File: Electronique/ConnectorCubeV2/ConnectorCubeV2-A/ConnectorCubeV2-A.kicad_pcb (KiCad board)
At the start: 2 copper layers, 95.2 x 95.2 mm, 133 parts, among them J1001 Conn_02x20_Odd_Even, J1002 Conn_02x20_Odd_Even, J1003 Conn_01x03, J1004 Conn_01x03, J1005 Conn_01x03, J1006 Conn_01x03, J1007 Conn_01x03, J1008 Conn_01x03, J1009 Conn_01x03, J1010 Conn_01x03, J1011 Conn_01x03, J1012 Conn_01x03, J1013 Conn_01x03, J201 Conn_01x04, J202 Conn_01x04, J203 Conn_01x04, J301 Conn_02x08_Odd_Even, J302 Conn_02x10_Odd_Even, J401 Conn_01x03, J402 Conn_01x03, J403 Conn_01x03, J404 Conn_01x03, J405 Conn_01x03, J501 Conn_01x04, J601 Conn_01x06, J602 Conn_01x06, J603 Conn_01x06, J801 Conn_01x02, J802 Conn_01x02, J901 Conn_01x04, J902 Conn_01x04, J903 Conn_01x04, K701 CONN_3, K702 CONN_3, Q301 BSS123, Q302 BSS123, Q303 BSS123, Q304 BSS123, Q305 BS250, Q401 BSS123, Q402 BSS123, Q403 BSS123, Q404 BSS123, Q405 BSS123, Q601 BSS123, Q602 BSS123, Q603 BSS123, Q604 BSS123, Q605 BSS123, Q606 BSS123, Q901 BSS123, Q902 BSS123, Q903 BSS123, U201 PCA9306, U202 PCA9306, U203 PCA9306, U301 74LVCC3245

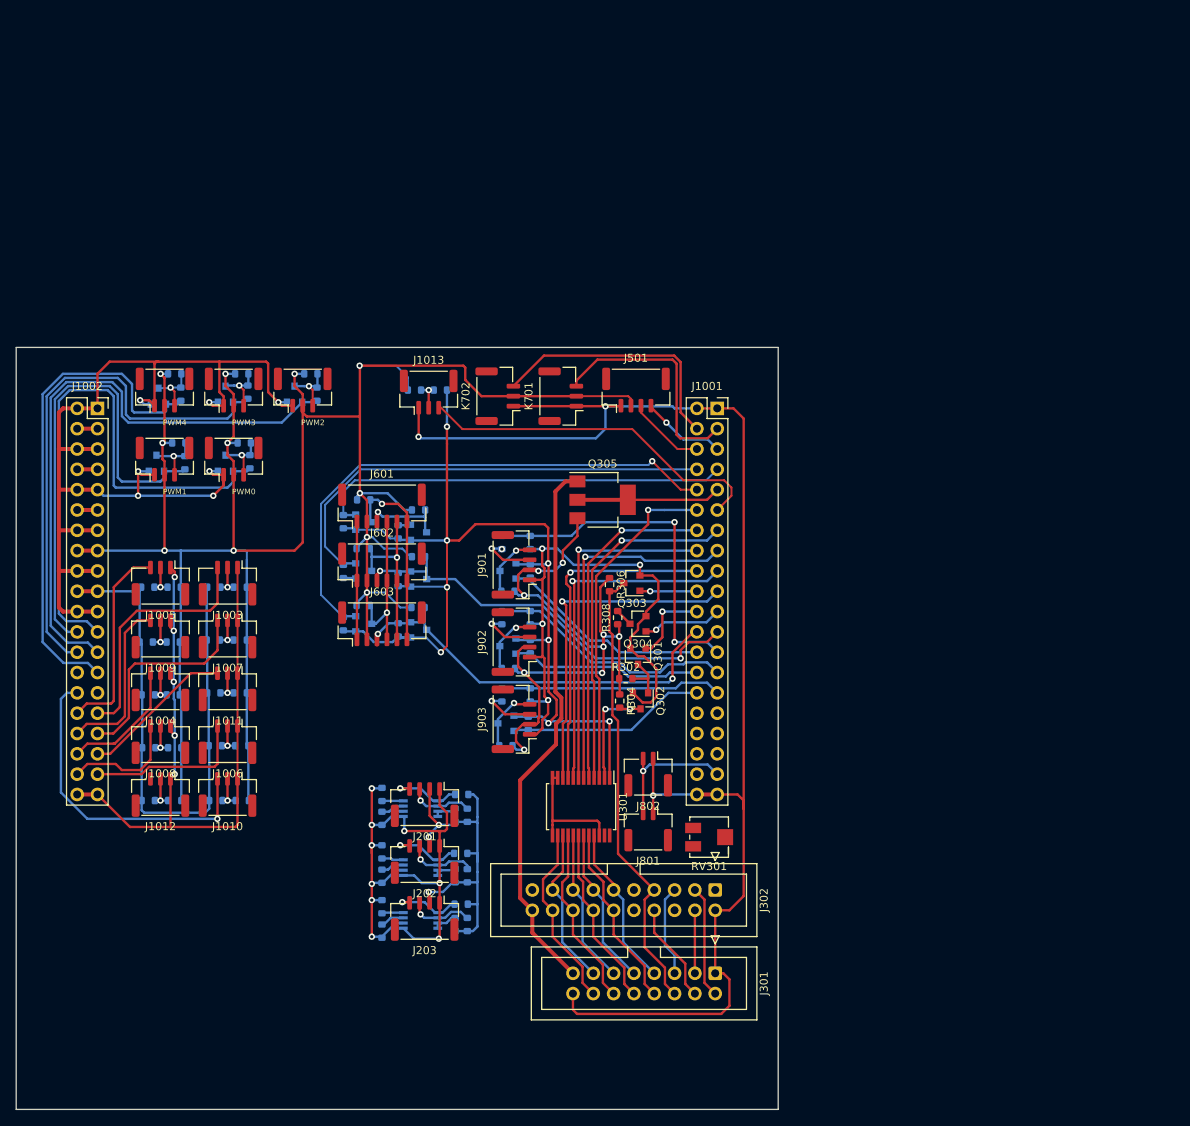
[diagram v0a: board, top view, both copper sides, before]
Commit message: CONNECTOR BOARD V2.00
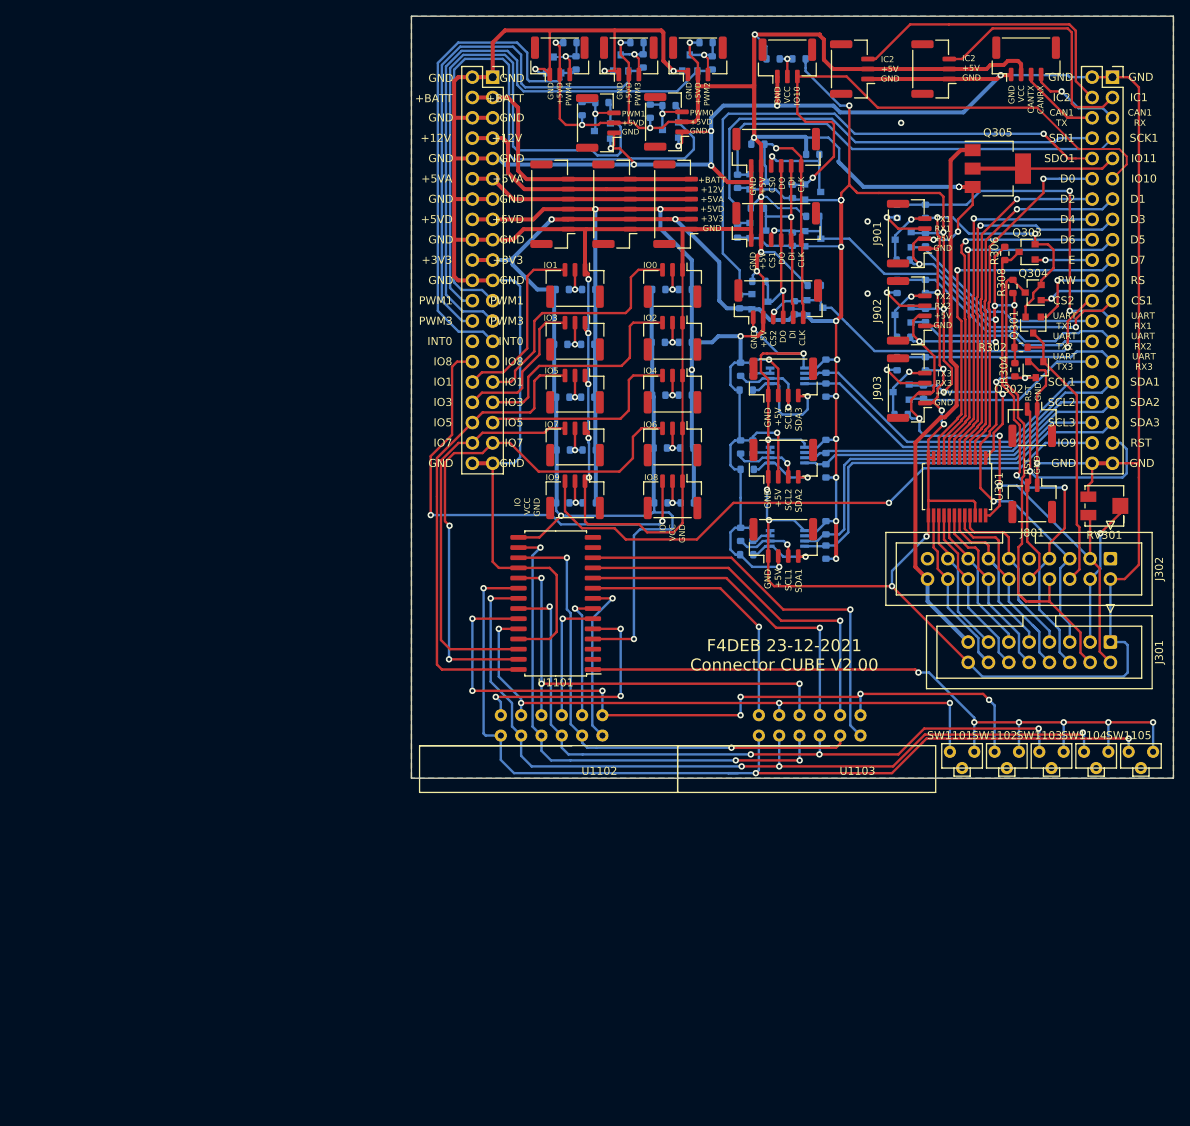
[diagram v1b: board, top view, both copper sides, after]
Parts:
- added J1201: Conn_01x06, Connector_JST:JST_GH_BM06B-GHS-TBT_1x06-1MP_P1.25mm_Vertical, F.Cu at (110.0, 75.3)
- added J1202: Conn_01x06, Connector_JST:JST_GH_BM06B-GHS-TBT_1x06-1MP_P1.25mm_Vertical, F.Cu at (117.7, 75.3)
- added J1203: Conn_01x06, Connector_JST:JST_GH_BM06B-GHS-TBT_1x06-1MP_P1.25mm_Vertical, F.Cu at (125.3, 75.3)
- added SW1101: SW_PUSH_SMALL, F4DEB-LIBRARY-KICAD5:BOUTON_SWITCH_4.5x4.5_angled, F.Cu at (159.6, 143.8)
- added SW1102: SW_PUSH_SMALL, F4DEB-LIBRARY-KICAD5:BOUTON_SWITCH_4.5x4.5_angled, F.Cu at (165.2, 143.8)
- added SW1103: SW_PUSH_SMALL, F4DEB-LIBRARY-KICAD5:BOUTON_SWITCH_4.5x4.5_angled, F.Cu at (170.8, 143.8)
- added SW1104: SW_PUSH_SMALL, F4DEB-LIBRARY-KICAD5:BOUTON_SWITCH_4.5x4.5_angled, F.Cu at (176.4, 143.8)
- added SW1105: SW_PUSH_SMALL, F4DEB-LIBRARY-KICAD5:BOUTON_SWITCH_4.5x4.5_angled, F.Cu at (182.0, 143.8)
- added U1101: TM1638, Package_SO:SOIC-28W_7.5x17.9mm_P1.27mm, F.Cu at (110.4, 125.2)
- added U1102: CA56-12EWA, F4DEB-LIBRARY-KICAD5:2841BS, F.Cu at (93.3, 143.0)
- added U1103: CA56-12EWA, F4DEB-LIBRARY-KICAD5:2841BS, F.Cu at (125.6, 143.0)
- R1001, R1002, R1003, R1004, R1005, R1007, R1009, R1010, R1011, R1012, R1013, R1014, R1015, R1016, R1017, R1018, R1019, R1020, R1021, R1022: value R -> 0
- moved R204 79.2 mm to (144.1, 95.6), turned to 270 degrees
- moved R205 77.2 mm to (144.1, 105.6), turned to 270 degrees
- moved R201 75.1 mm to (144.1, 98.6), turned to 90 degrees
- moved R206 75.0 mm to (144.1, 115.8), turned to 270 degrees
- moved R202 73.1 mm to (144.1, 108.6), turned to 90 degrees
- moved R203 71.0 mm to (144.1, 118.8), turned to 90 degrees
- moved U201 70.9 mm to (139.3, 96.8), turned to 180 degrees
- moved Q402 69.5 mm to (116.2, 66.2), turned to 180 degrees
- moved Q401 69.5 mm to (124.7, 66.0), turned to 180 degrees
- moved J201 69.5 mm to (138.8, 97.3), turned to 0 degrees
- moved U202 69.0 mm to (139.3, 106.7), turned to 180 degrees
- moved R402 68.9 mm to (116.1, 62.6), turned to 180 degrees
- moved R401 68.7 mm to (124.5, 63.0), turned to 180 degrees
- moved J402 68.6 mm to (115.7, 65.2), turned to 90 degrees
- moved J401 68.6 mm to (124.2, 65.0), turned to 90 degrees
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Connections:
- J1001 pad 33: (no net) -> /SDA2
- Q604 pad 2: /SCS -> /IO10
- R202 pad 2: /I2C/SDA2 -> /SDA2
- R604 pad 2: /SCS -> /IO10
- U202 pad 4: /I2C/SDA2 -> /SDA2
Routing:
- net GND: track 545.7 -> 795.3 mm, vias 22 -> 32
- net +5VD: track 423.9 -> 566.2 mm, vias 23 -> 30
- net /7Seg/E: track 0.00 -> 116.5 mm, vias 0 -> 3
- net /7Seg/D: track 0.00 -> 103.6 mm, vias 0 -> 4
- net +3V3: track 247.0 -> 348.2 mm, vias 14 -> 19
- net /7Seg/B: track 0.00 -> 94.6 mm, vias 0 -> 7
- net /7Seg/K1: track 0.00 -> 91.5 mm, vias 0 -> 6
- net /7Seg/C: track 0.00 -> 88.9 mm, vias 0 -> 4
- net /IO9: track 0.00 -> 76.1 mm, vias 0 -> 1
- net /7Seg/A: track 0.00 -> 75.6 mm, vias 0 -> 4
- net /7Seg/DOT: track 0.00 -> 64.9 mm, vias 0 -> 3
- net /7Seg/G: track 0.00 -> 63.7 mm, vias 0 -> 2
- net /7Seg/F: track 0.00 -> 56.2 mm, vias 0 -> 3
- net /7Seg/S8: track 0.00 -> 51.1 mm, vias 0 -> 1
- net /LCD/BRS: track 14.7 -> 62.6 mm
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- added copper zone on B.Cu, net GND
- added copper zone on F.Cu, net GND
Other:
- board size 95.2 x 95.2 mm -> 95.3 x 95.2 mm
- board text added: "+12V"
- board text added: "+3.3V"
- board text added: "+3V3"
- board text added: "+5V"
- board text added: "+5VA"
- board text added: "+5VD"
- board text added: "+BATT"
- board text added: "+BATT +12V +5VA +5VD +3V3 GND"
- board text added: "3.3V"
- board text added: "CAN1 RX"
- board text added: "CAN1 TX"
- board text added: "CS1"
- board text added: "CS2"
- board text added: "D0"
- board text added: "D1"
- board text added: "D2"
- board text added: "D3"
- board text added: "D4"
- board text added: "D5"
- board text added: "D6"
- board text added: "D7"
- board text added: "E"
- board text added: "F4DEB 23-12-2021 Connector CUBE V2.00"
- board text added: "GND"
- board text added: "GND +5V CS0 DO DI CLK"
- board text added: "GND +5V CS1 DO DI CLK"
- board text added: "GND +5V CS2 DO DI CLK"
- board text added: "GND +5V SCL1 SDA1"
- board text added: "GND +5V SCL2 SDA2"
- board text added: "GND +5V SCL3 SDA3"
- board text added: "GND +5VD PWM2"
- board text added: "GND +5VD PWM3"
- board text added: "GND +5VD PWM4"
- board text added: "GND BD7 BD5 BD3 BD1 BE BRS +5V"
- board text added: "GND VCC CANTX CANRX"
- board text added: "GND VCC IO10"
- board text added: "IC1"
- board text added: "IC2"
- board text added: "IC2 +5V GND"
- board text added: "INT0"
- board text added: "IO VCC GND"
- board text added: "IO0"
- board text added: "IO1"
- board text added: "IO10"
- board text added: "IO11"
- board text added: "IO2"
- board text added: "IO3"
- board text added: "IO4"
- board text added: "IO5"
- board text added: "IO6"
- board text added: "IO7"
- board text added: "IO8"
- board text added: "IO9"
- board text added: "PWM0 +5VD GND"
- board text added: "PWM1 +5VD GND"
- board text added: "RS"
- board text added: "RST"
- board text added: "RST GND"
- board text added: "RW"
- board text added: "SCK1"
- board text added: "SCL1"
- board text added: "SCL2"
- board text added: "SCL3"
- board text added: "SDA1"
- board text added: "SDA2"
- board text added: "SDA3"
- board text added: "SDI1"
- board text added: "SDO1"
- board text added: "TX1 RX1 +5V GND"
- board text added: "TX2 RX2 +5V GND"
- board text added: "TX3 RX3 +5V GND"
- board text added: "UART RX1"
- board text added: "UART RX2"
- board text added: "UART RX3"
- board text added: "UART TX1"
- board text added: "UART TX2"
- board text added: "UART TX3"
- board text removed: "PWM0"
- board text removed: "PWM2"
- board text removed: "PWM4"

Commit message: reprise 28-7-2022
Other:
- net class Default removed
